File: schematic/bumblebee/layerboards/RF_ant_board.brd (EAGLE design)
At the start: 36 x 30 mm, 2 parts, among them J1 U.FL-R-SMT(01)

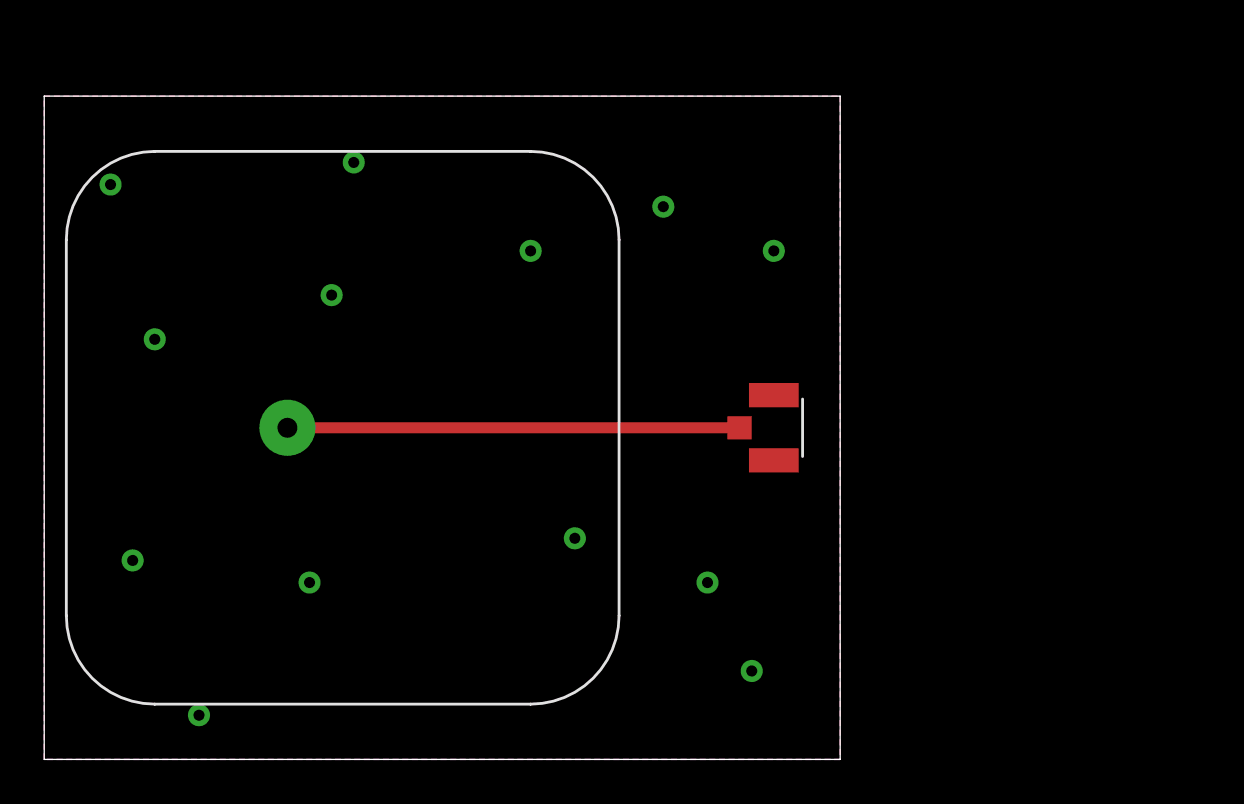
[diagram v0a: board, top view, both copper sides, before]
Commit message: Все платы готовы и отправлены в Резонит
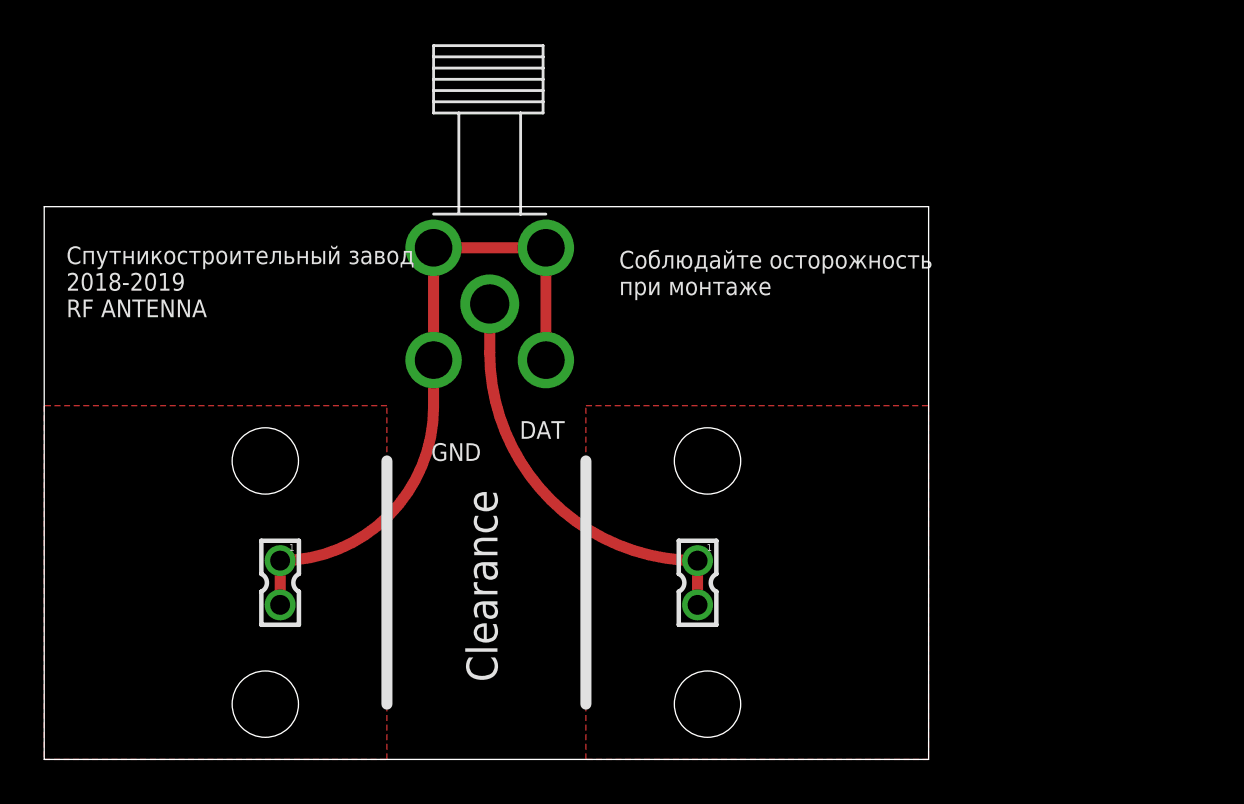
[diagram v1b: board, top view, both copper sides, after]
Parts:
- removed U$1: BY-IRIDIUM-254, iridium-antenna:BY-IRIDIUM-254
- added X1, X2: 332-02, con-garry:332-02
- J1: value U.FL-R-SMT(01) -> 221790-1; device U.FL-R-SMT_01_:HRS_U.FL-R-SMT(01) -> 221790-1:TE_221790-1
- moved J1 14.0 mm to (20.1, 20.6), turned to 90 degrees
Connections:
- removed net N$1: J1.3, U$1.P$1
- new net DAT: J1.1, X1.1, X1.2
- net GND: now also J1.3, J1.4, J1.5, X2.1, X2.2; no longer J1.1
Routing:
- net GND: track 0.00 -> 29.2 mm, vias 13 -> 0
- net N$1: track 20.4 -> 0.00 mm
- net DAT: track 0.00 -> 17.5 mm
- added copper zone on layer 1, net DAT
- removed copper zone on layer 16, net GND
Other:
- board size 36 x 30 mm -> 40 x 25 mm
- board text added: "Clearance"
- board text added: "DAT"
- board text added: "GND"
- board text added: "Соблюдайте осторожность при монтаже"
- board text added: "Спутникостроительный завод 2018-2019 RF ANTENNA"
